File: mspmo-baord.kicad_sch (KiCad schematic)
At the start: 37 parts, among them J1 USB_C_Receptacle_USB2.0_16P, J2 Conn_ARM_SWD_TagConnect_TC2030, U1 SPX3819M5-L-3-3, U3 MSPM0G3507SPTR, U4 CH340E, U5 LIS2DH, X1 8MHz

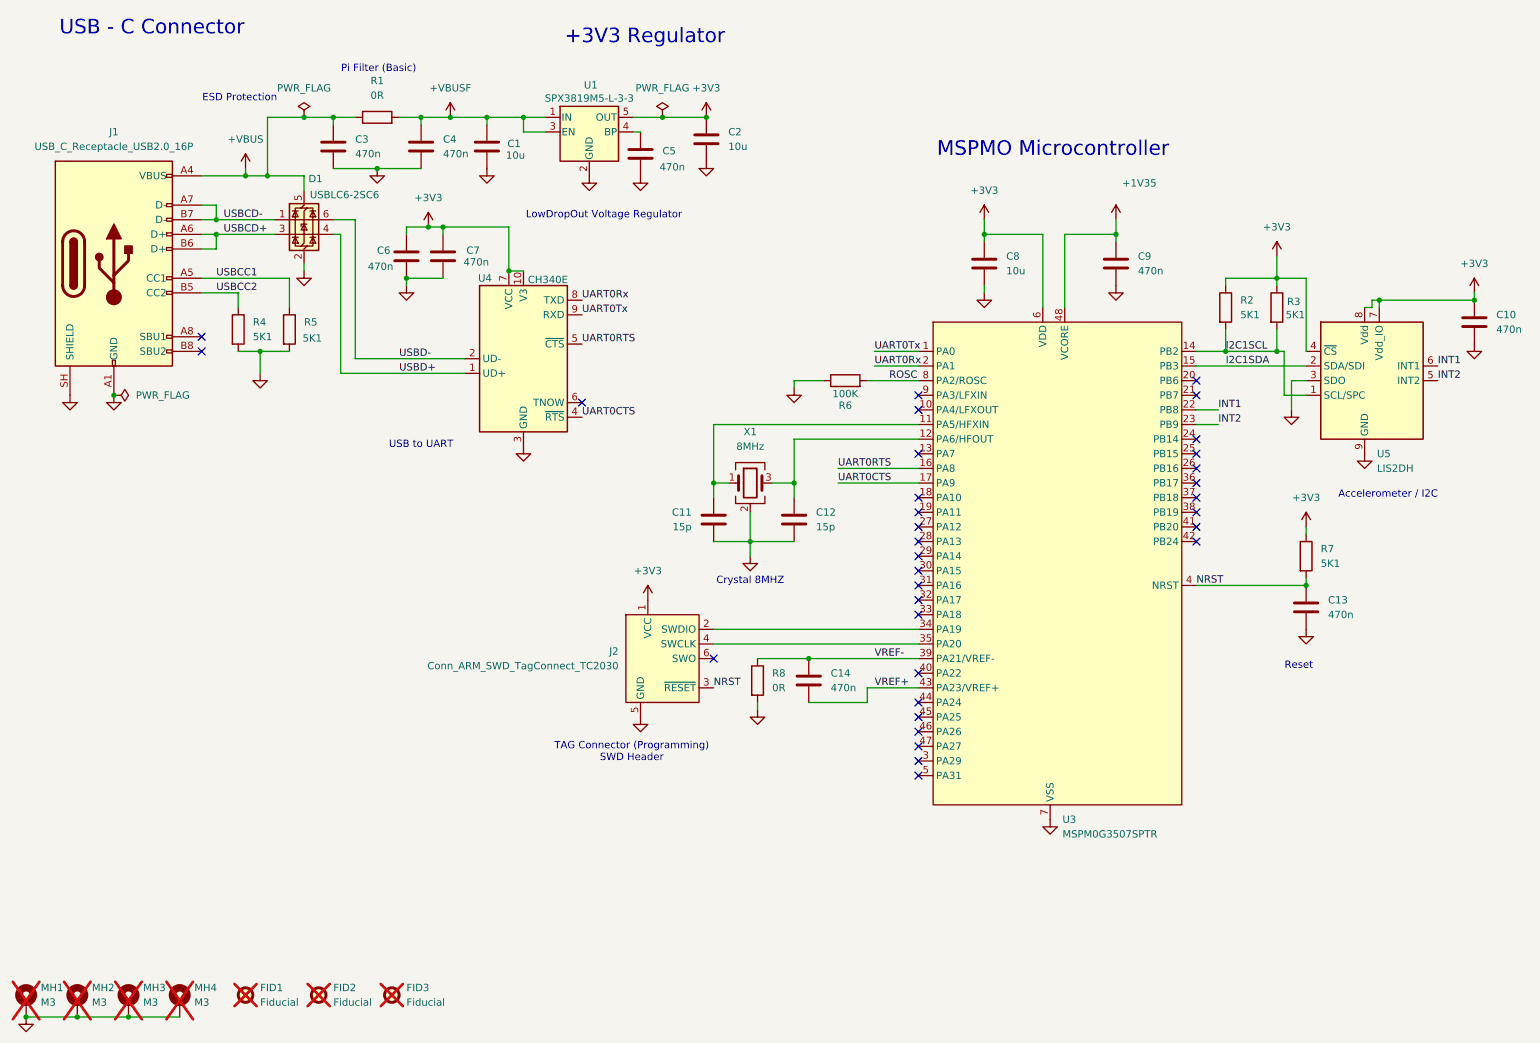
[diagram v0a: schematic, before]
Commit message: pcb files
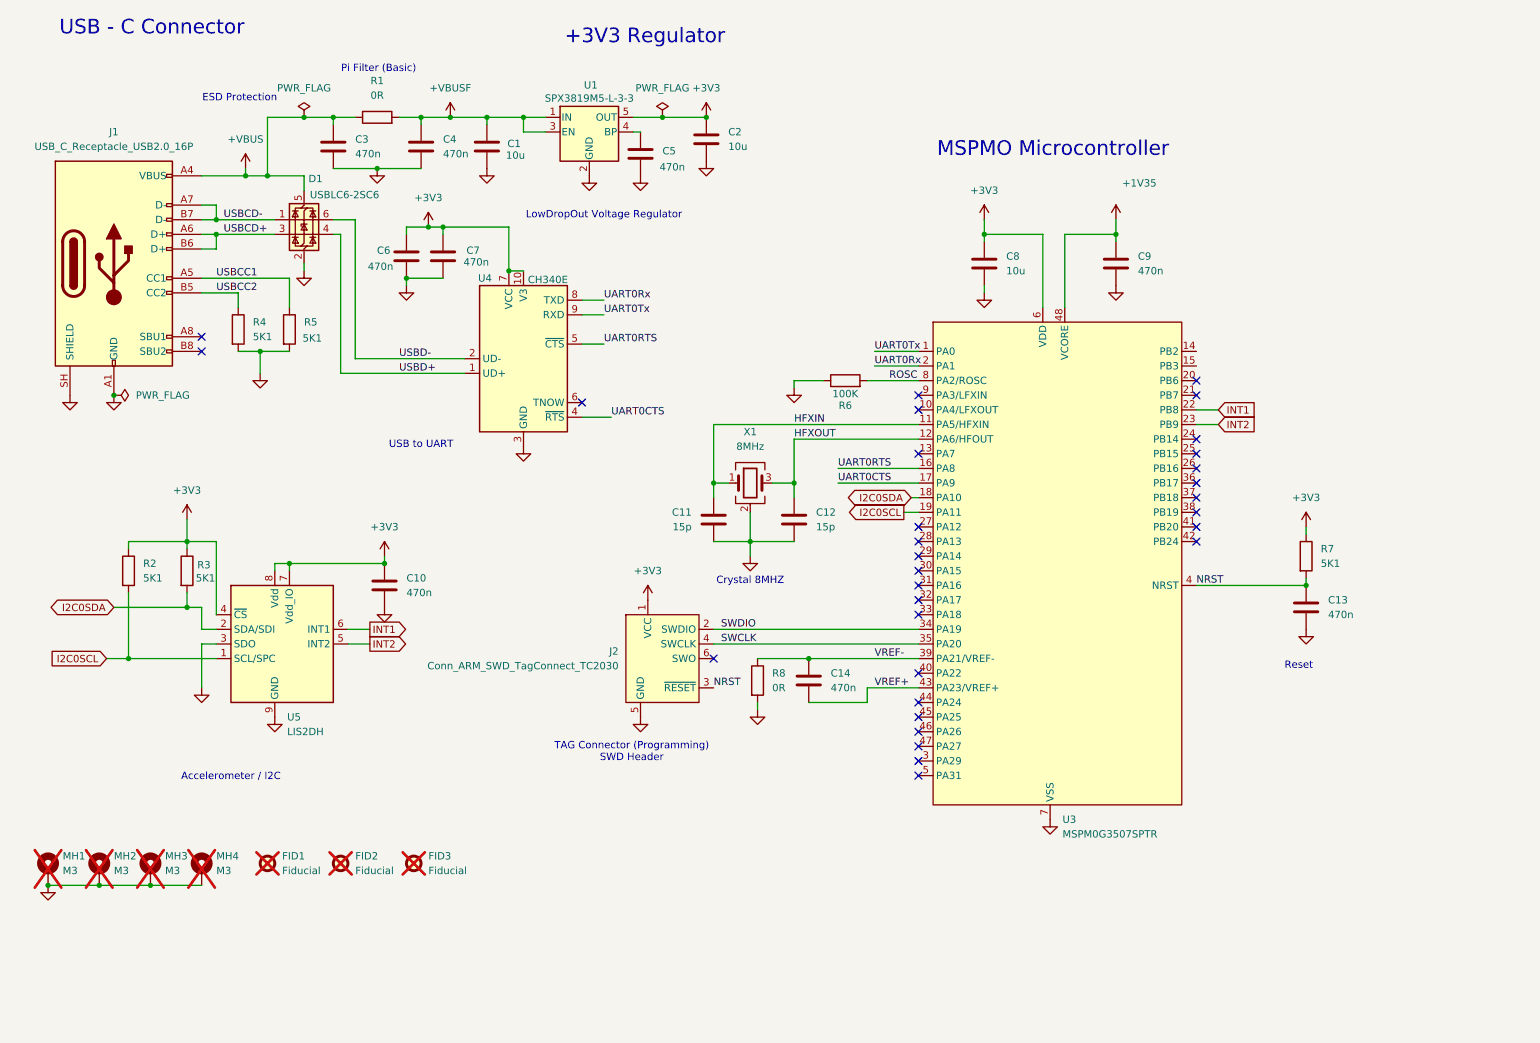
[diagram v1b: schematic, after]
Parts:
- R1, R2, R3, R4, R5, R6, R7, R8: footprint Resistor_SMD:R_0201_0603Metric -> Resistor_SMD:R_0603_1608Metric
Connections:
- net SWDIO: now reaches J2.2 (SWDIO), U3.34 (PA19)
- net SWCLK: now reaches J2.4 (SWCLK), U3.35 (PA20)
- net HFXOUT: now reaches C12.1, U3.12 (PA6/HFOUT), X1.3
- net HFXIN: now reaches C11.1, U3.11 (PA5/HFXIN), X1.1
- net I2C0SDA: now reaches U3.18 (PA10)
- net I2C0SDA: now also R3.2, U5.2 (SDA/SDI)
- net I2C0SCL: now reaches U3.19 (PA11)
- net I2C0SCL: now also R2.2, U5.1 (SCL/SPC)
- removed net I2C1SCL: R2.2, R3.2, U3.14 (PB2), U5.1 (SCL/SPC)
- net I2C1SDA: no longer names the net of U3.15 (PB3)
- net I2C1SDA: no longer U5.2 (SDA/SDI)
- no-connect marks 33 -> 31
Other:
- moved on the sheet: C10, FID1, FID2, FID3, MH1, MH2, MH3, MH4, R2, R3, U5
